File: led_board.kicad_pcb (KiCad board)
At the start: 2 copper layers, 12 parts, among them J1 Conn_Coaxial, J2 Conn_Coaxial, J3 Conn_Coaxial, J4 Conn_Coaxial

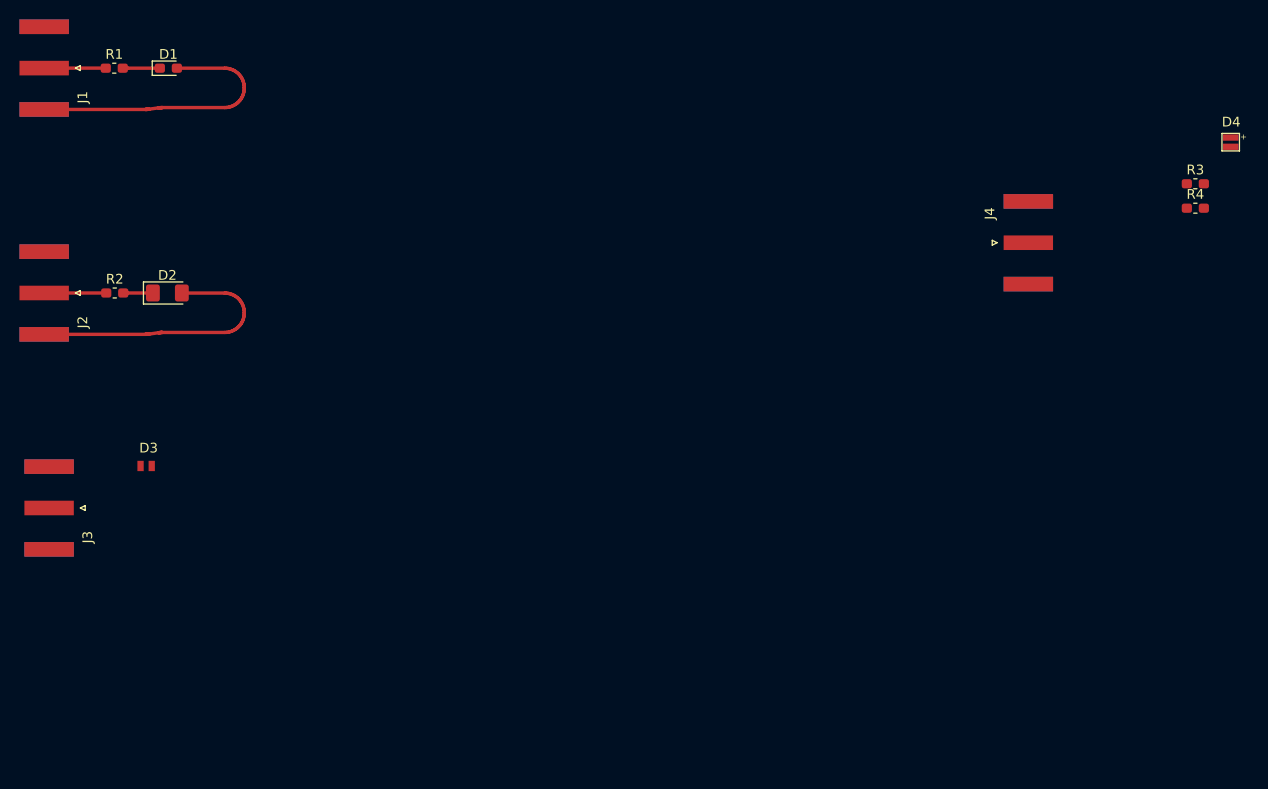
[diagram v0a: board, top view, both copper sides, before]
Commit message: edits
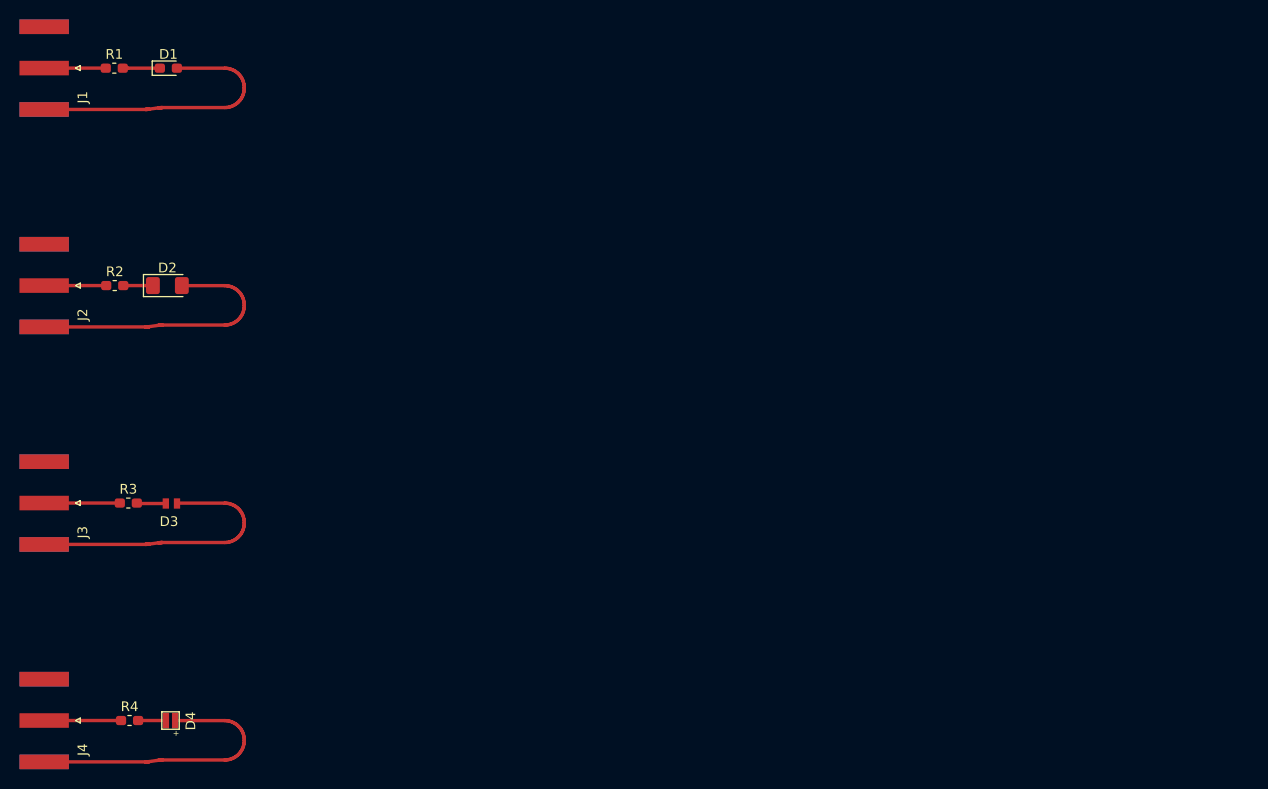
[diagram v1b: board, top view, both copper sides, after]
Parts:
- moved D4 124.5 mm to (52.5, 109.7), turned to 270 degrees
- moved R4 121.5 mm to (49.2, 109.7)
- moved R3 114.5 mm to (49.0, 87.4)
- moved J4 112.4 mm to (40.4, 109.7), turned to 180 degrees
- moved D3 6.88 mm to (53.2, 88.8), turned to 0 degrees
- moved D2 0.76 mm to (53.0, 65.0)
- moved J2 0.76 mm to (40.4, 65.0)
- moved R2 0.76 mm to (47.6, 65.0)
- moved J3 0.72 mm to (40.4, 87.4)
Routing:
- net Net-(D3-Pad2): track 0.00 -> 29.8 mm
- net Net-(D4-Pad2): track 0.00 -> 29.8 mm
- net Net-(J4-Pad1): track 0.00 -> 7.90 mm
- net Net-(J3-Pad1): track 0.00 -> 7.77 mm
- net Net-(D3-Pad1): track 0.00 -> 3.00 mm
- net Net-(D4-Pad1): track 0.00 -> 2.86 mm
